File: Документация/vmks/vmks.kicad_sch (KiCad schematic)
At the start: 6 parts

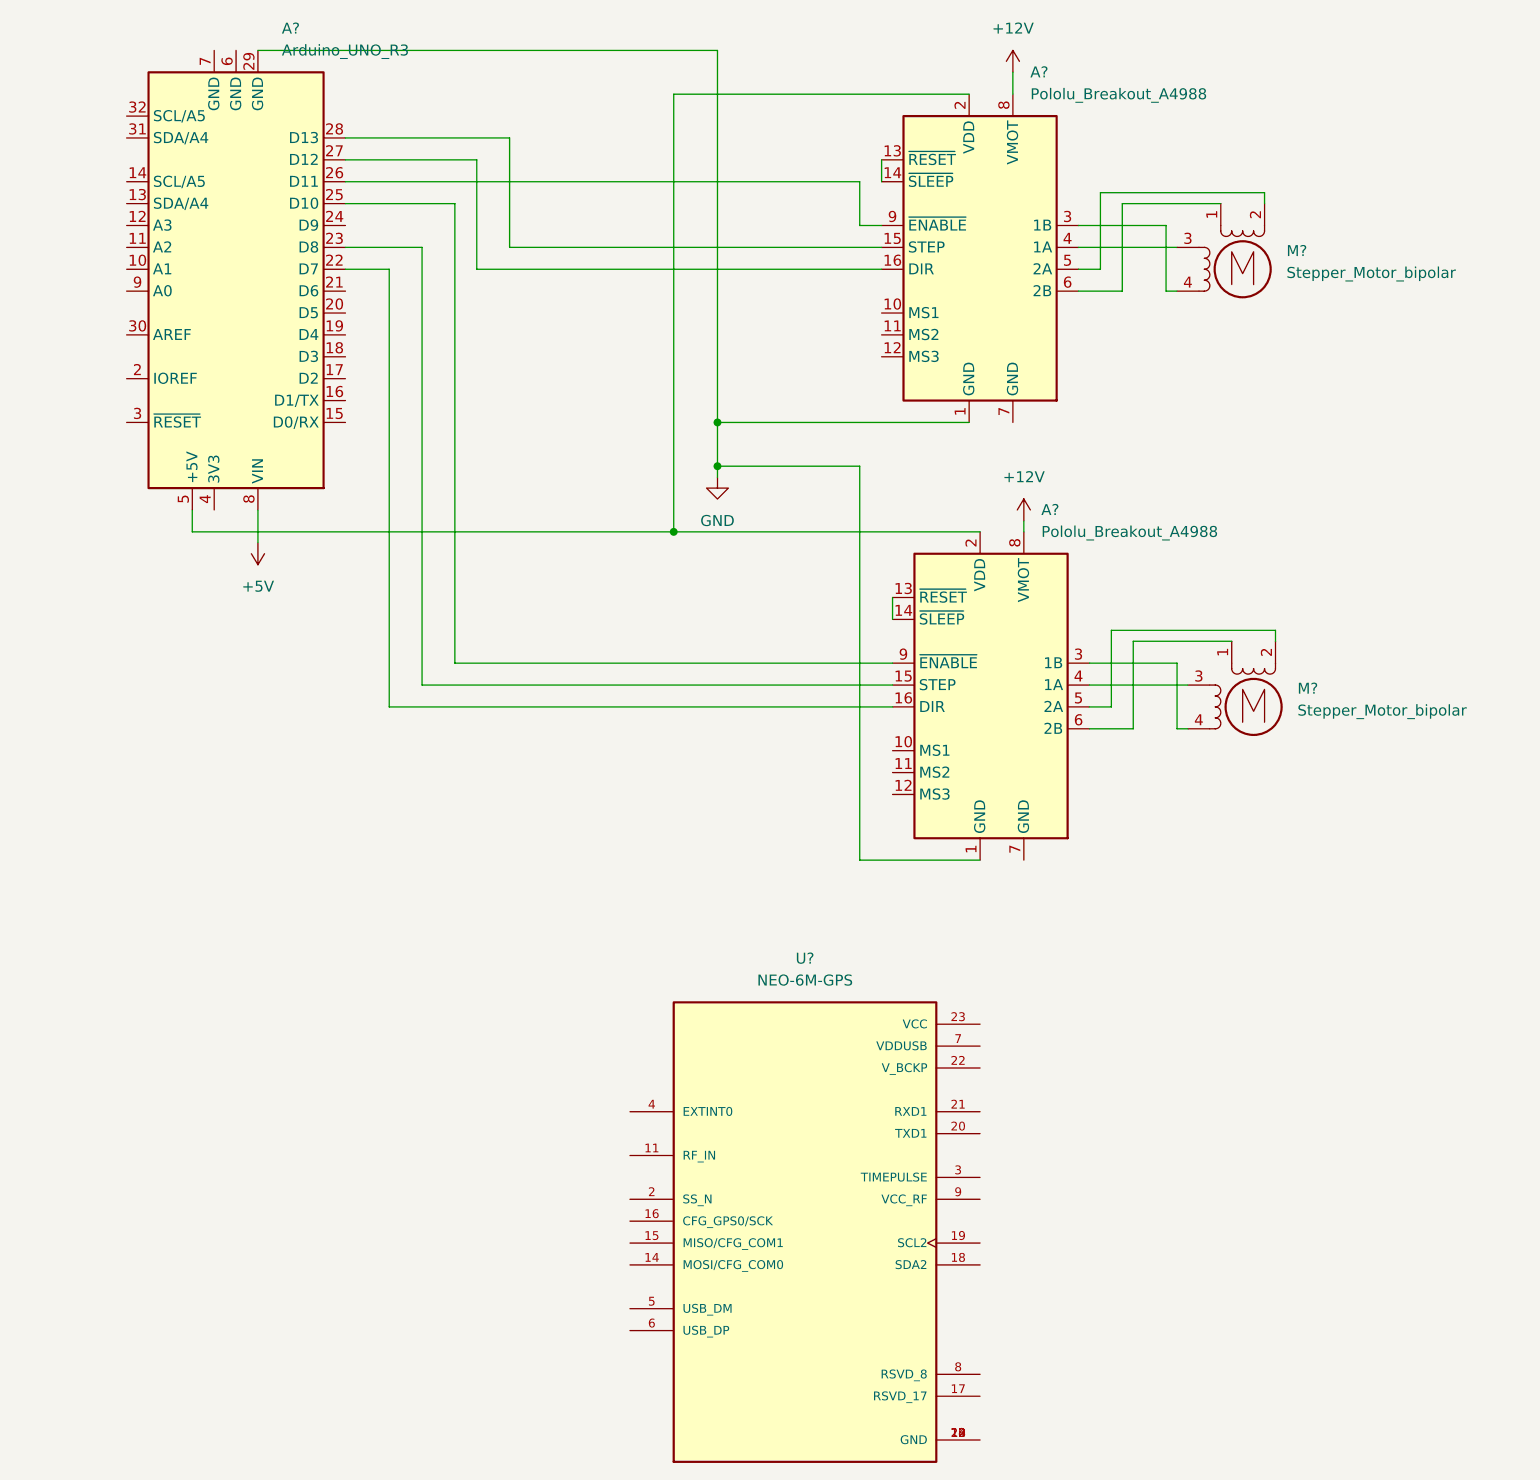
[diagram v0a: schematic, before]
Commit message: updated schematic
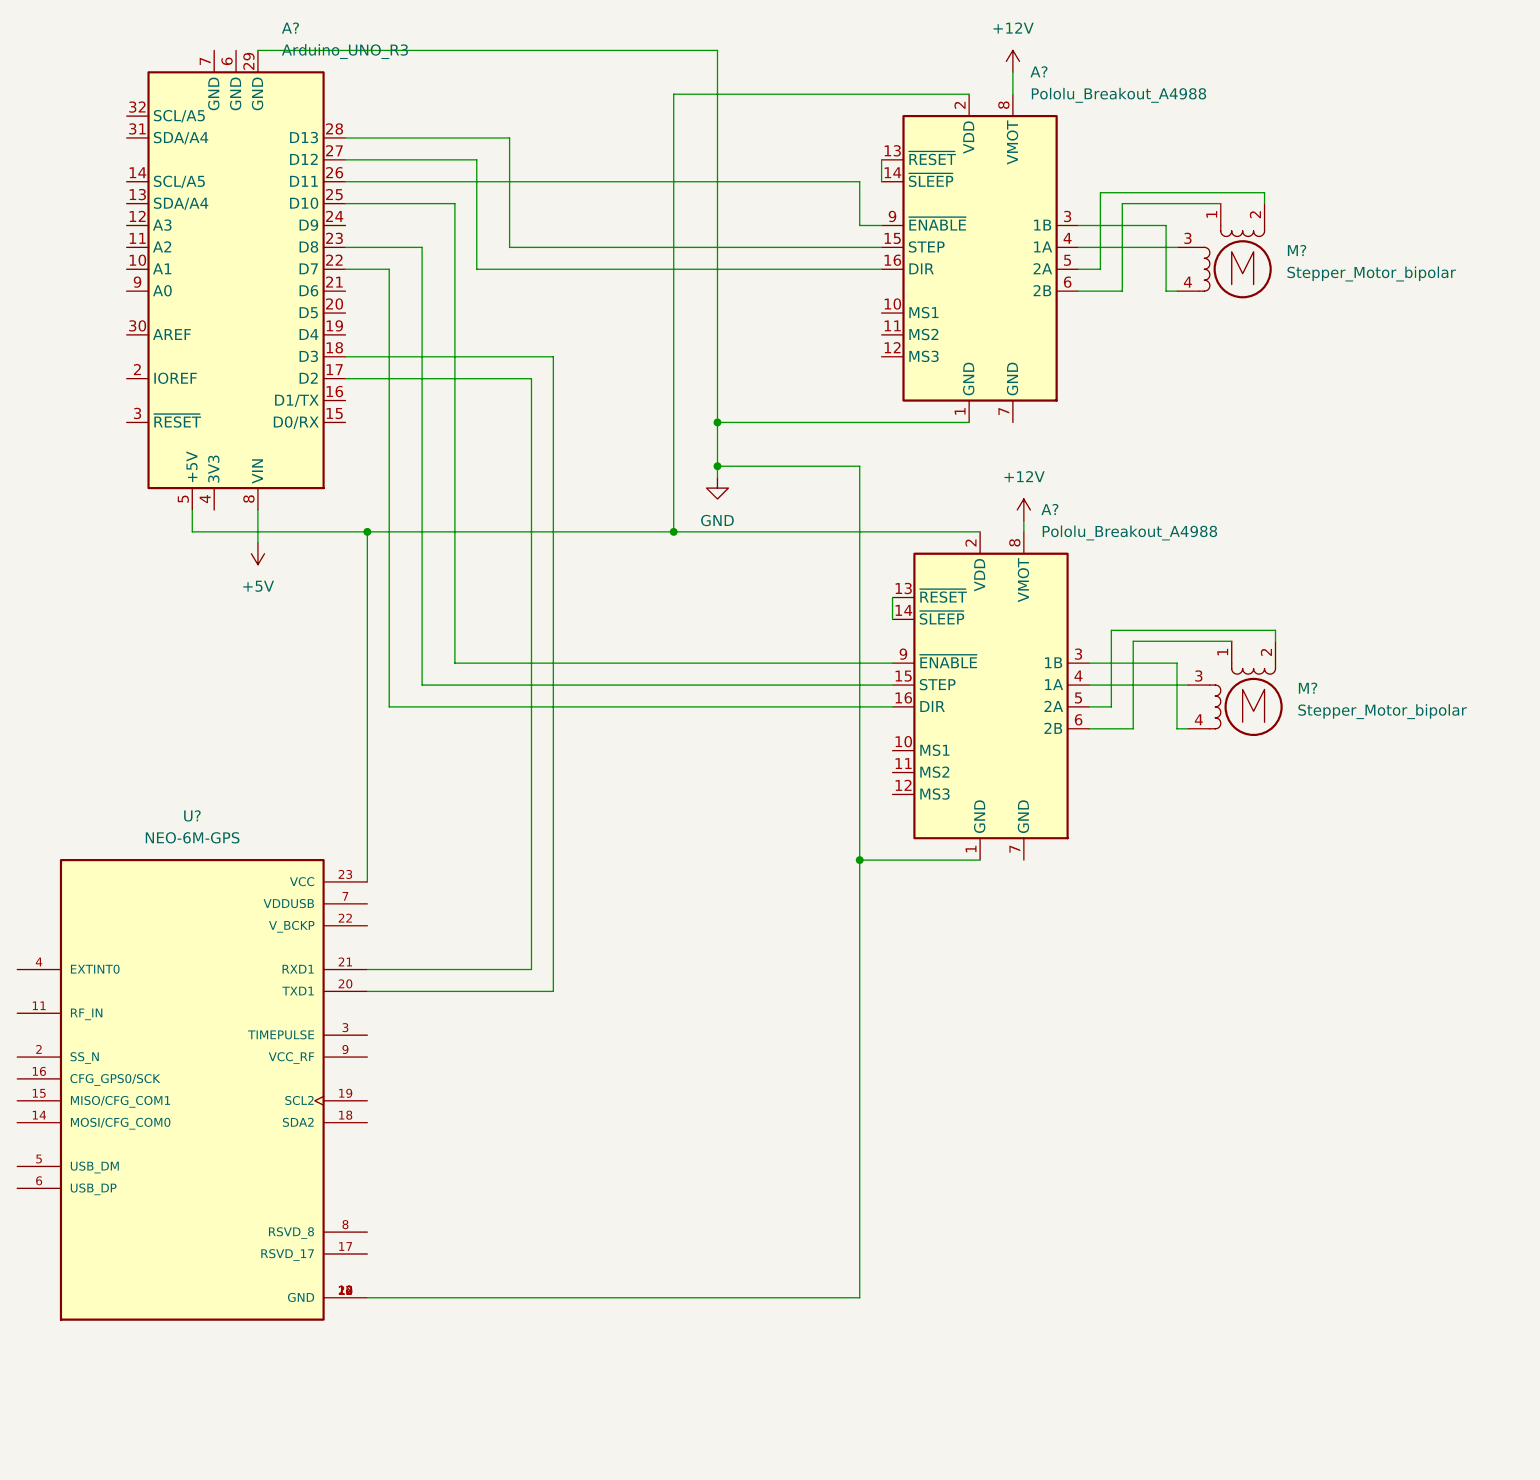
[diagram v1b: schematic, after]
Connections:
- net GND: now also U?.10 (GND), U?.12 (GND), U?.13 (GND), U?.24 (GND)
- net at A?.2 (VDD), A?.2 (VDD), A?.5 (+5V): now also U?.23 (VCC)
- net at U?.20 (TXD1): now also A?.18 (D3)
- net at U?.21 (RXD1): now also A?.17 (D2)
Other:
- moved on the sheet: U?
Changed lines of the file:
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@@
   (junction (at 135.89 73.66) (diameter 0) (color 0 0 0 0)
   )
+  (junction (at 95.25 81.28) (diameter 0) (color 0 0 0 0)
+  )
   (junction (at 130.81 81.28) (diameter 0) (color 0 0 0 0)
   )
+  (junction (at 152.4 119.38) (diameter 0) (color 0 0 0 0)
+  )
   (wire (pts (xy 189.23 96.52) (xy 189.23 104.14))
     (stroke (width 0) (type default) (color 0 0 0 0))
@@
     (stroke (width 0) (type default) (color 0 0 0 0))
   )
+  (wire (pts (xy 95.25 81.28) (xy 130.81 81.28))
+    (stroke (width 0) (type default) (color 0 0 0 0))
+  )
+  (wire (pts (xy 95.25 132.08) (xy 114.3 132.08))
+    (stroke (width 0) (type default) (color 0 0 0 0))
+  )
   (wire (pts (xy 189.23 104.14) (xy 190.5 104.14))
     (stroke (width 0) (type default) (color 0 0 0 0))
@@
     (stroke (width 0) (type default) (color 0 0 0 0))
   )
+  (wire (pts (xy 114.3 63.5) (xy 92.71 63.5))
+    (stroke (width 0) (type default) (color 0 0 0 0))
+  )
+  (wire (pts (xy 95.25 134.62) (xy 116.84 134.62))
+    (stroke (width 0) (type default) (color 0 0 0 0))
+  )
   (wire (pts (xy 200.66 93.98) (xy 200.66 92.71))
     (stroke (width 0) (type default) (color 0 0 0 0))
@@
     (stroke (width 0) (type default) (color 0 0 0 0))
   )
+  (wire (pts (xy 95.25 170.18) (xy 152.4 170.18))
+    (stroke (width 0) (type default) (color 0 0 0 0))
+  )
   (wire (pts (xy 180.34 41.91) (xy 180.34 50.8))
     (stroke (width 0) (type default) (color 0 0 0 0))
@@
     (stroke (width 0) (type default) (color 0 0 0 0))
   )
+  (wire (pts (xy 116.84 134.62) (xy 116.84 60.96))
+    (stroke (width 0) (type default) (color 0 0 0 0))
+  )
   (wire (pts (xy 184.15 93.98) (xy 195.58 93.98))
     (stroke (width 0) (type default) (color 0 0 0 0))
@@
     (stroke (width 0) (type default) (color 0 0 0 0))
   )
-  (wire (pts (xy 74.93 81.28) (xy 130.81 81.28))
+  (wire (pts (xy 74.93 81.28) (xy 95.25 81.28))
+    (stroke (width 0) (type default) (color 0 0 0 0))
+  )
+  (wire (pts (xy 152.4 170.18) (xy 152.4 119.38))
     (stroke (width 0) (type default) (color 0 0 0 0))
   )
@@
     (stroke (width 0) (type default) (color 0 0 0 0))
   )
+  (wire (pts (xy 116.84 60.96) (xy 92.71 60.96))
+    (stroke (width 0) (type default) (color 0 0 0 0))
+  )
   (wire (pts (xy 135.89 73.66) (xy 135.89 74.93))
     (stroke (width 0) (type default) (color 0 0 0 0))
@@
   )
   (wire (pts (xy 107.95 38.1) (xy 92.71 38.1))
+    (stroke (width 0) (type default) (color 0 0 0 0))
+  )
+  (wire (pts (xy 114.3 132.08) (xy 114.3 63.5))
+    (stroke (width 0) (type default) (color 0 0 0 0))
+  )
+  (wire (pts (xy 95.25 81.28) (xy 95.25 121.92))
     (stroke (width 0) (type default) (color 0 0 0 0))
   )
@@
     (pin "1")
   )
-  (symbol (lib_id "RF_GPS:NEO-6M-GPS") (at 146.05 161.29 0) (unit 1)
-    (in_bom yes) (on_board yes) (fields_autoplaced)
-    (property "Reference" "U?" (id 0) (at 146.05 130.81 0))
-    (property "Value" "NEO-6M-GPS" (id 1) (at 146.05 133.35 0))
-    (property "Footprint" "XCVR_NEO-6M-GPS" (id 2) (at 146.05 161.29 0)
+  (symbol (lib_id "RF_GPS:NEO-6M-GPS") (at 74.93 144.78 0) (unit 1)
+    (in_bom yes) (on_board yes) (fields_autoplaced)
+    (property "Reference" "U?" (id 0) (at 74.93 114.3 0))
+    (property "Value" "NEO-6M-GPS" (id 1) (at 74.93 116.84 0))
+    (property "Footprint" "XCVR_NEO-6M-GPS" (id 2) (at 74.93 144.78 0)
       (effects (font (size 1.27 1.27)) (justify bottom) hide)
     )
-    (property "Datasheet" "" (id 3) (at 146.05 161.29 0)
-      (effects (font (size 1.27 1.27)) hide)
-    )
-    (property "STANDARD" "Manufacturer Recommendations" (id 4) (at 146.05 161.29 0)
+    (property "Datasheet" "" (id 3) (at 74.93 144.78 0)
+      (effects (font (size 1.27 1.27)) hide)
+    )
+    (property "STANDARD" "Manufacturer Recommendations" (id 4) (at 74.93 144.78 0)
       (effects (font (size 1.27 1.27)) (justify bottom) hide)
     )
-    (property "PARTREV" "R15" (id 5) (at 146.05 161.29 0)
+    (property "PARTREV" "R15" (id 5) (at 74.93 144.78 0)
       (effects (font (size 1.27 1.27)) (justify bottom) hide)
     )
-    (property "MANUFACTURER" "U-Blox" (id 6) (at 146.05 161.29 0)
+    (property "MANUFACTURER" "U-Blox" (id 6) (at 74.93 144.78 0)
       (effects (font (size 1.27 1.27)) (justify bottom) hide)
     )
